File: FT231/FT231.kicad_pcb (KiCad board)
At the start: 2 copper layers, 20.3 x 15.5 mm, 21 parts, among them J1 USB_B_Micro, J2 Conn_01x03, J3 Conn_01x03, J4 Conn_01x06, U1 FT231XQ

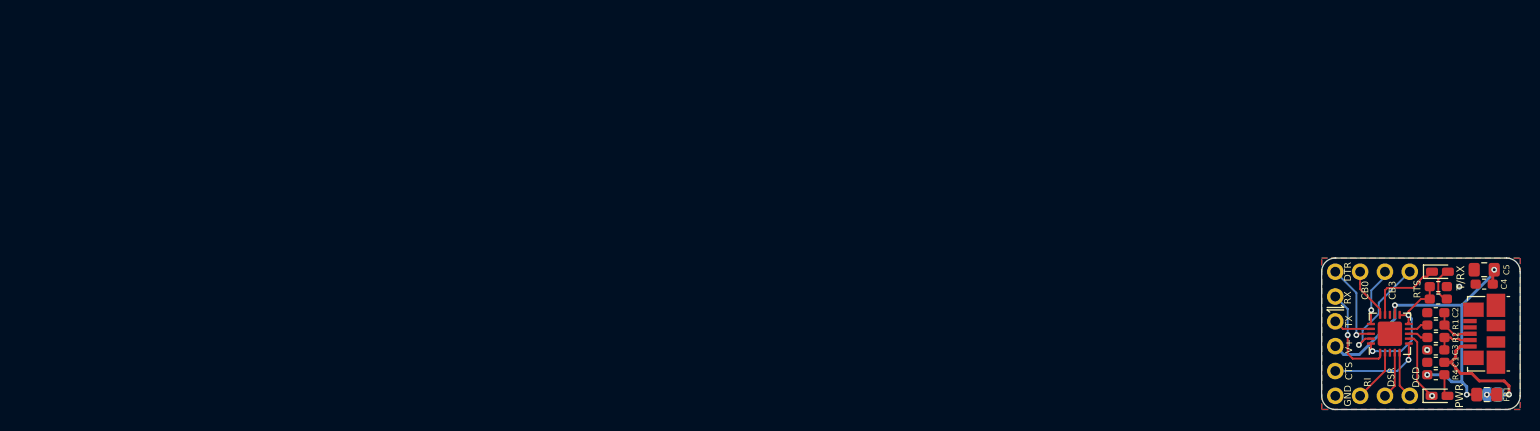
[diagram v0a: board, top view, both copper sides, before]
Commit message: Page Settings Updated
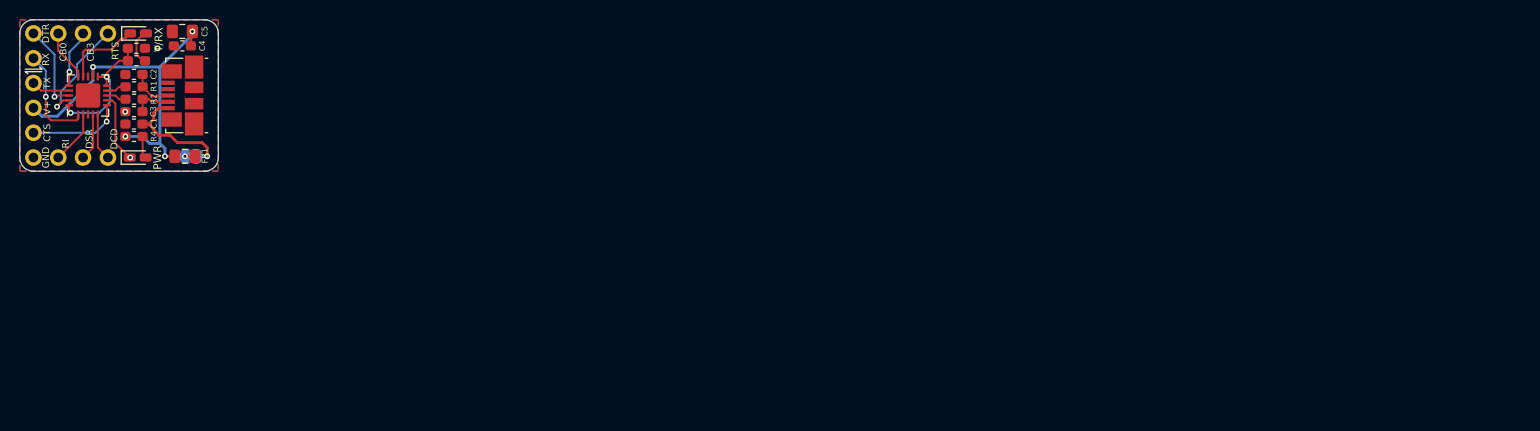
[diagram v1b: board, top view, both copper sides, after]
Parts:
- moved C1 135.4 mm to (70.1, 45.8)
- moved C2 135.4 mm to (70.1, 40.8)
- moved C3 135.4 mm to (70.1, 44.6)
- moved C4 135.4 mm to (75.1, 37.8)
- moved C5 135.4 mm to (75.1, 36.4)
- moved FB1 135.4 mm to (75.3, 49.1)
- moved G*** 135.4 mm to (65.5, 42.9)
- moved J1 135.4 mm to (75.1, 42.9)
- moved J2 135.4 mm to (62.4, 49.3)
- moved J3 135.4 mm to (62.4, 36.6)
- moved JP1 135.4 mm to (75.9, 49.1)
- moved PWR 135.4 mm to (70.5, 49.3)
- moved R1 135.4 mm to (70.1, 42.0)
- moved R2 135.4 mm to (70.1, 43.3)
- moved R4 135.4 mm to (70.1, 47.1)
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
